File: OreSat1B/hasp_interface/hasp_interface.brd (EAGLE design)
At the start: 83 x 100 mm, 79 parts, among them J1 SAMTEC-MMS-104-02-X-SHJ, J2 ORESAT-DEBUG-CONNECTOR-ALL, Q1 MMBT2907SMD, U1 TCAN330, U10 TPS63070, U2 LM60440ARPKR, U7 STM32F091C, X1 16MHZ-2.5x2mm

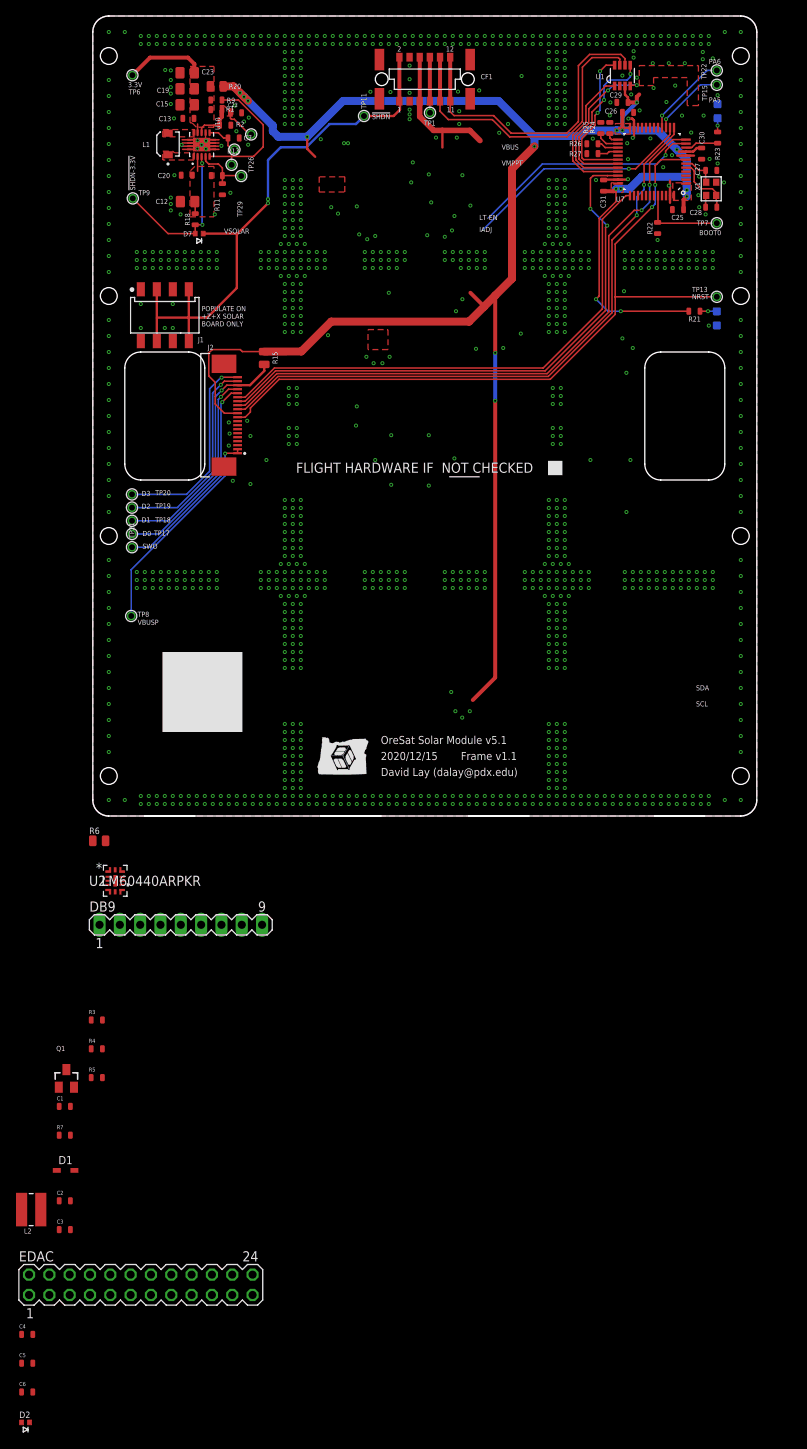
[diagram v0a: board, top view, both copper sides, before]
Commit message: Wire cleanup
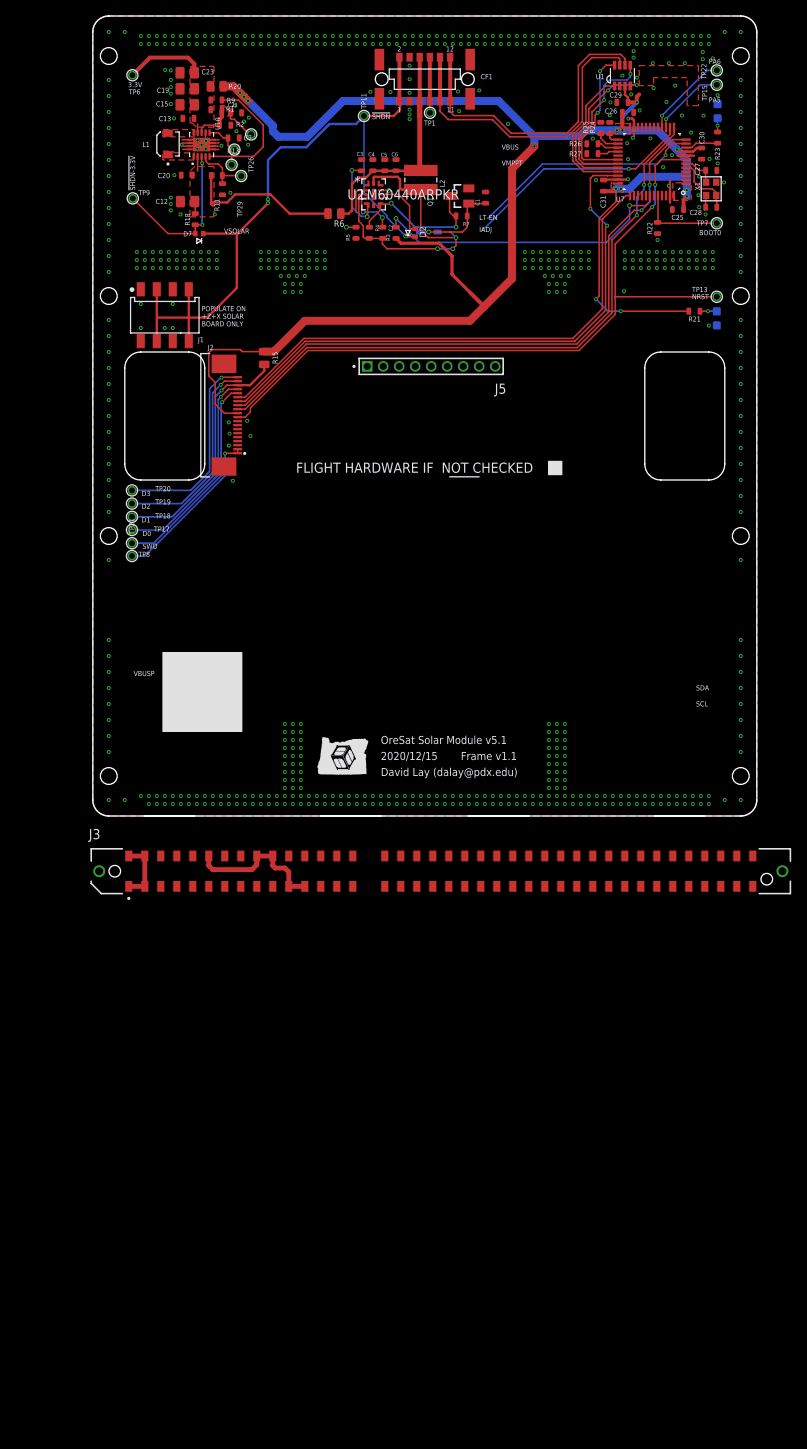
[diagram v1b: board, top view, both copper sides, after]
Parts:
- removed DB9: (no value), con-lstb:MA09-1
- removed EDAC: (no value), con-lstb:MA12-2
- added J3: MEC2-40-01-X-DV-WT, MEC2-40-01-X-DV-WT:SAMTEC_MEC2-40-01-X-DV-WT
- added J5: TW-09-03-G-S-245-145, TW-09-03-G-S-245-145:SAMTEC_TW-09-03-G-S-245-145
- moved C6 160.1 mm to (37.9, 81.3), turned to 90 degrees
- moved D2 156.5 mm to (40.3, 72.9), turned to 270 degrees
- moved C5 156.3 mm to (36.5, 81.3), turned to 90 degrees
- moved C4 152.4 mm to (35.0, 81.3), turned to 90 degrees
- moved C3 138.1 mm to (33.6, 81.3), turned to 90 degrees
- moved L2 137.6 mm to (41.0, 79.5), turned to 90 degrees
- moved C2 127.4 mm to (36.2, 72.9), turned to 270 degrees
- moved D1 125.8 mm to (42.0, 73.0), flipped to the bottom
- moved C1 125.2 mm to (49.1, 77.3), turned to 90 degrees
- moved R7 125.1 mm to (46.1, 75.0), turned to 180 degrees
- moved Q1 120.8 mm to (45.9, 77.5), turned to 90 degrees
- moved R5 110.5 mm to (32.9, 72.9), turned to 90 degrees
- moved R4 107.5 mm to (34.6, 72.9), turned to 270 degrees
- moved R3 105.3 mm to (37.9, 72.9), turned to 90 degrees
- moved U2 91.7 mm to (35.1, 77.7)
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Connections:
- net +30VDC: now also J3.01, J3.02, J3.03, J3.04; no longer EDAC.1, EDAC.2, EDAC.3, EDAC.4
- net GND: now also J3.12, J3.18, J3.20, J3.21, J3.23; no longer EDAC.12, EDAC.18, EDAC.20, EDAC.21, EDAC.23
- net TURNSTILEFIRE-(DISCRETE1): now also J3.06; no longer EDAC.6
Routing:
- net 3.3V: track 259.1 -> 217.9 mm, vias 17 -> 14
- net N$7: track 0.00 -> 40.7 mm, vias 0 -> 3
- net TURNSTILEFIRE-(DISCRETE1): track 0.00 -> 38.2 mm, vias 0 -> 2
- net N$2: track 0.00 -> 19.9 mm, vias 0 -> 3
- net TPS-VIN: track 3.38 -> 23.2 mm
- net !SHUTDOWN: track 72.6 -> 91.0 mm, vias 2 -> 3
- net GND: track 21.1 -> 39.2 mm, vias 1197 -> 653
- net +30VDC: track 0.00 -> 12.6 mm, vias 0 -> 1
- net N$4: track 0.00 -> 11.3 mm, vias 0 -> 1
- net VBUS: track 18.3 -> 28.4 mm
- net N$6: track 0.00 -> 9.93 mm, vias 0 -> 2
- net N$8: track 0.00 -> 7.75 mm
- net N$1: track 27.2 -> 20.6 mm
- net N$5: track 0.00 -> 6.25 mm, vias 0 -> 2
- removed copper zone on layer 1, net VSOLAR
